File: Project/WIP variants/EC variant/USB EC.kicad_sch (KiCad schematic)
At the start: 6 parts, among them J1 USB_C_Receptacle_USB2.0, U2 PRTR5V0U2X

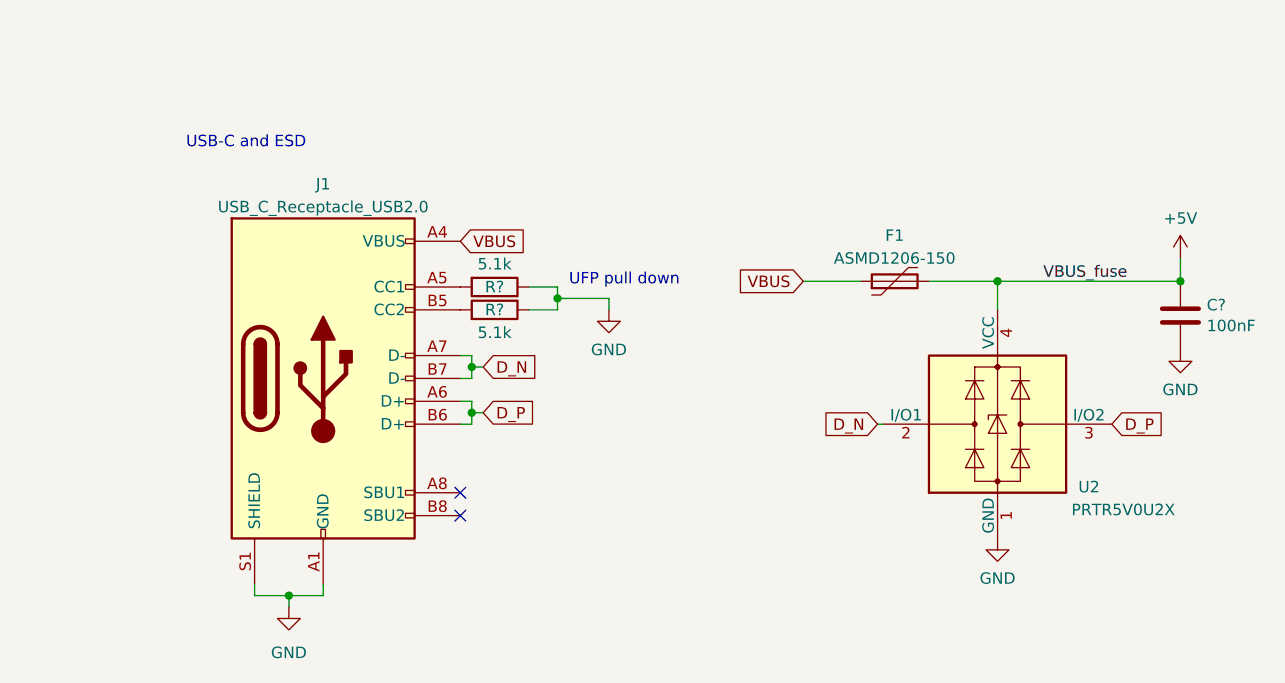
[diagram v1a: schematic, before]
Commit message: BLE & EC edited
requires production files!!
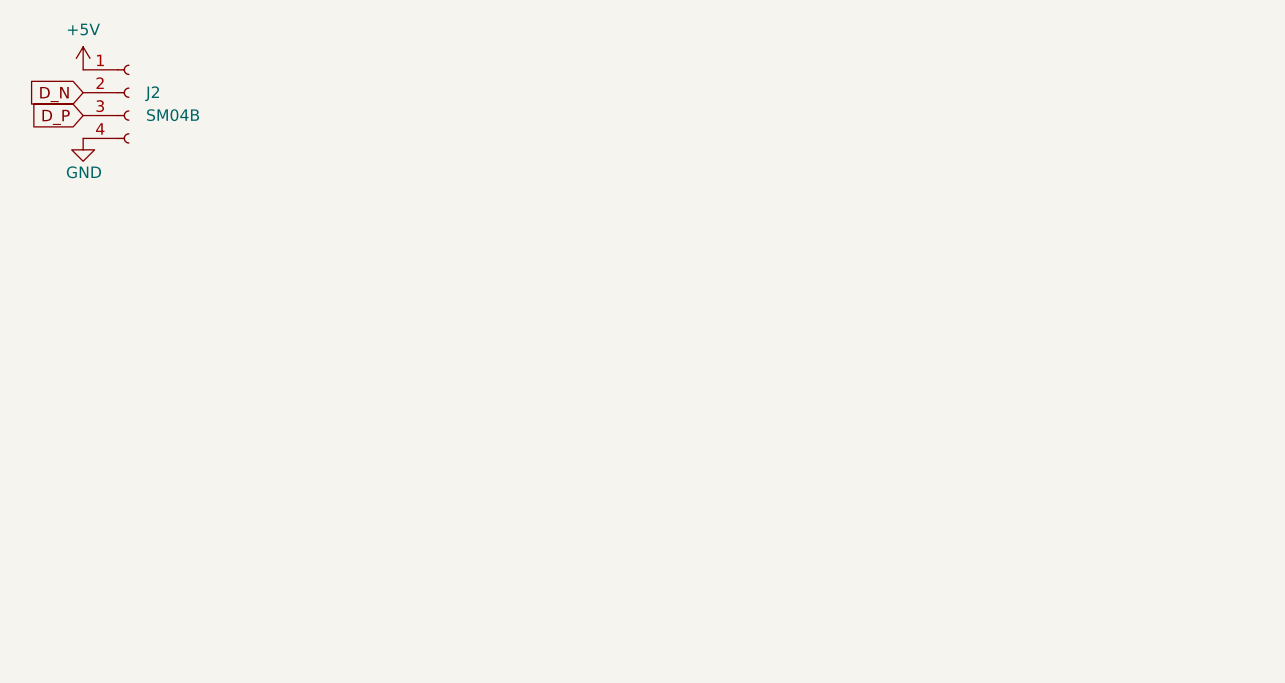
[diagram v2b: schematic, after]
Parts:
- removed C?: 100nF, Capacitor_SMD:C_0402_1005Metric, symbol Device:C
- removed F1: ASMD1206-150, Fuse:Fuse_1206_3216Metric, symbol Device:Polyfuse
- removed J1: USB_C_Receptacle_USB2.0, Connector_USB:USB_C_Receptacle_HRO_TYPE-C-31-M-12, symbol Connector:USB_C_Receptacle_USB2.0
- removed R? (x2): 5.1k, Resistor_SMD:R_0402_1005Metric, symbol Device:R
- removed U2: PRTR5V0U2X, Package_TO_SOT_SMD:SOT-143, symbol Power_Protection:PRTR5V0U2X
- added J2: SM04B, Connector_JST:JST_SH_SM04B-SRSS-TB_1x04-1MP_P1.00mm_Horizontal, symbol Connector:Conn_01x04_Female
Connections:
- net +5V: now also J2.1 (Pin_1)
- net D_N: now also J2.2 (Pin_2)
- net D_P: now also J2.3 (Pin_3)
- net GND: now also J2.4 (Pin_4)
- no-connect marks 2 -> 0
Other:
- note removed: "UFP pull down"
- note removed: "USB-C and ESD"
